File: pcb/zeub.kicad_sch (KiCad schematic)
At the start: 39 parts, among them J1 debug-port, J2 OLED-128x32, J5 Conn_01x03, J6 Conn_01x03, J7 Micro_SD_Card_Det, Q1 AO3400A, Q2 AO3400A, Q3 AO3400A, Q4 AO3400A, Q5 AO3400A, Q6 AO3401A, Q7 AO3401A, Q8 AO3401A, Q9 AO3401A, SW1 SKRHA, SW2 RotaryEncoder_Switch, SW3 SW_Push, U11 TMP117, U5 holyiot-18010-no-underside, U6 MT25QL128ABA1ESE

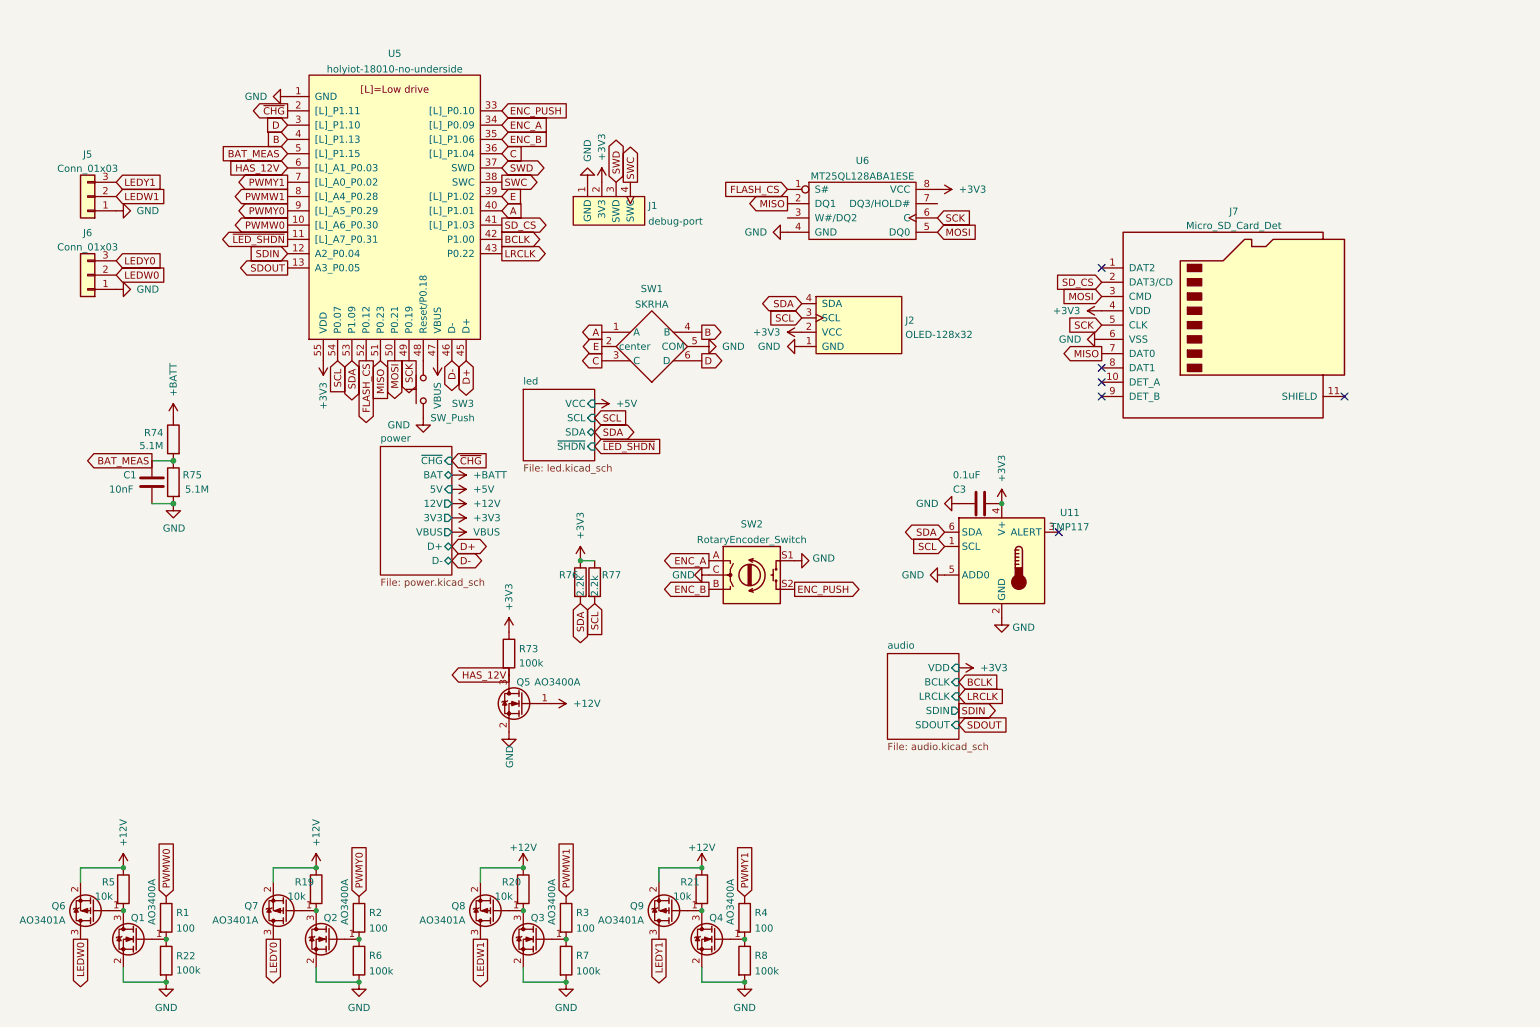
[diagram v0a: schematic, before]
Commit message: v2
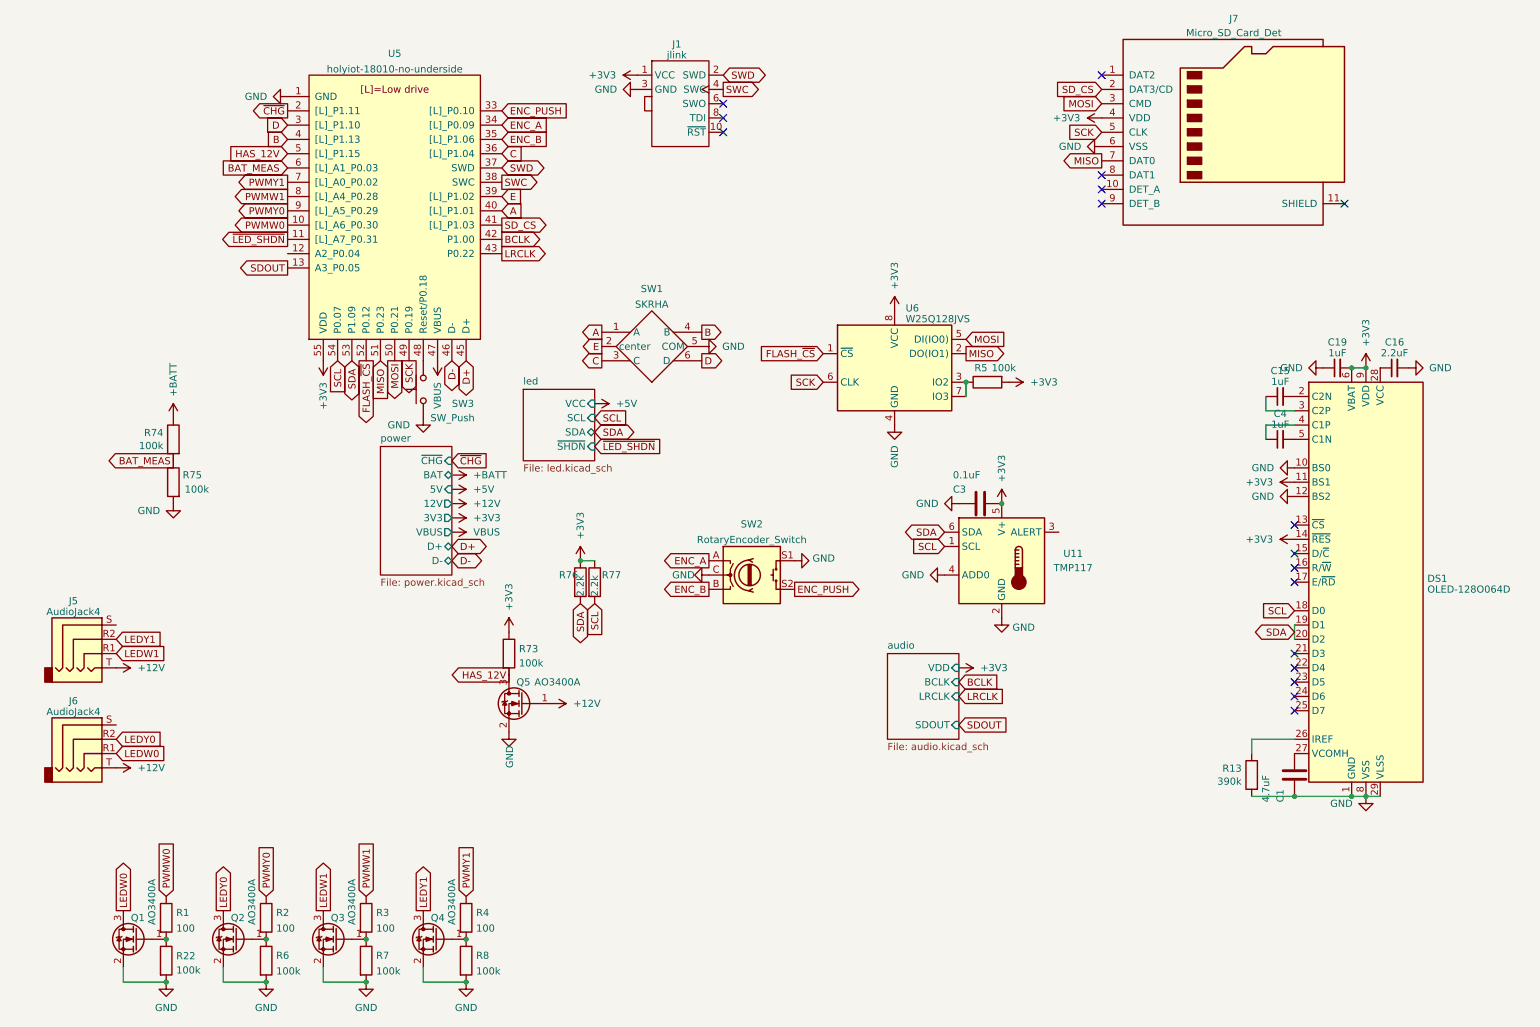
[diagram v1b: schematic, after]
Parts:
- removed J1: debug-port, misc:debug-port-single-side, symbol misc:debug-port
- removed J2: OLED-128x32, display:OLED-128x64, symbol display:OLED-128x32
- removed J5, J6: Conn_01x03, Connector_PinHeader_2.54mm:PinHeader_1x03_P2.54mm_Vertical, symbol Connector_Generic:Conn_01x03
- removed Q6, Q7, Q8, Q9: AO3401A, Package_TO_SOT_SMD:SOT-23, symbol Transistor_FET:AO3401A
- removed R19, R20, R21: 10k, Resistor_SMD:R_0603_1608Metric, symbol Device:R
- removed U6: MT25QL128ABA1ESE, Package_SO:SOIC-8_5.23x5.23mm_P1.27mm, symbol ic:MT25QL128ABA1ESE
- added C15, C19, C4: 1uF, Capacitor_SMD:C_0603_1608Metric, symbol Device:C_Small
- added C16: 2.2uF, Capacitor_SMD:C_0603_1608Metric, symbol Device:C_Small
- added DS1: OLED-128O064D, Display:OLED-128O064D, symbol Display_Graphic:OLED-128O064D
- added J1: jlink, Connector_PinHeader_1.27mm:PinHeader_2x05_P1.27mm_Vertical_SMD, symbol misc:jlink
- added J5, J6: AudioJack4, Connector_Audio:Jack_3.5mm_PJ320D_Horizontal, symbol Connector:AudioJack4
- added R13: 390k, Resistor_SMD:R_0603_1608Metric, symbol Device:R
- added U6: W25Q128JVS, Package_SO:SOIC-8_5.23x5.23mm_P1.27mm, symbol Memory_Flash:W25Q128JVS
- C1: value 10nF -> 4.7uF
- R5: value 10k -> 100k
- R74, R75: value 5.1M -> 100k
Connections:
- net +12V: now also J5.T, J6.T; no longer R5.1
- net +3V3: now also R5.2, U11.5 (V+), C19.2, DS1.11 (BS1), DS1.14 (~{RES}), DS1.6 (VBAT), DS1.9 (VDD), J1.1 (VCC), U6.8 (VCC); no longer U11.4 (V+)
- net BAT_MEAS: now also U5.6 ([L]_A1_P0.03); no longer C1.1, U5.5 ([L]_P1.15)
- net GND: now also C1.1, U11.4 (ADD0), C16.2, C19.1, DS1.1 (GND), DS1.10 (BS0), DS1.12 (BS2), DS1.29 (VLSS), DS1.30 (GND), DS1.8 (VSS), J1.3 (GND), J1.5 (GND), R13.2, U6.4 (GND); no longer C1.2, U11.5 (ADD0)
- net HAS_12V: now also U5.5 ([L]_P1.15); no longer U5.6 ([L]_A1_P0.03)
- net LEDW0: now also Q1.3 (D), J6.R1
- net LEDW1: now also Q3.3 (D), J5.R1
- net LEDY0: now also Q2.3 (D), J6.R2
- net LEDY1: now also Q4.3 (D), J5.R2
- net MISO: now also U6.2 (DO(IO1))
- net MOSI: now also U6.5 (DI(IO0))
- net SCK: now also U6.6 (CLK)
- net SCL: now also DS1.18 (D0)
- net SDA: now also DS1.19 (D1), DS1.20 (D2)
- net SWC: now also J1.4 (SWC)
- net SWD: now also J1.2 (SWD)
- net FLASH_CS renamed FLASH_~{CS}
- net FLASH_~{CS}: now also U6.1 (~{CS})
- net SDIN: no longer names the net of U5.12 (A2_P0.04)
- new net: R5.1, U6.3 (IO2), U6.7 (IO3)
- new net: C4.1, DS1.4 (C1P)
- new net: C4.2, DS1.5 (C1N)
- new net: C16.1, DS1.28 (VCC)
- new net: C1.2, DS1.27 (VCOMH)
- new net: C15.1, DS1.3 (C2P)
- new net: C15.2, DS1.2 (C2N)
- new net: DS1.26 (IREF), R13.1
- no-connect marks 6 -> 17
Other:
- sheet audio ports: added none; removed SDIN
- moved on the sheet: J7, Q2, Q3, Q4, R2, R3, R4, R6, R7, R8

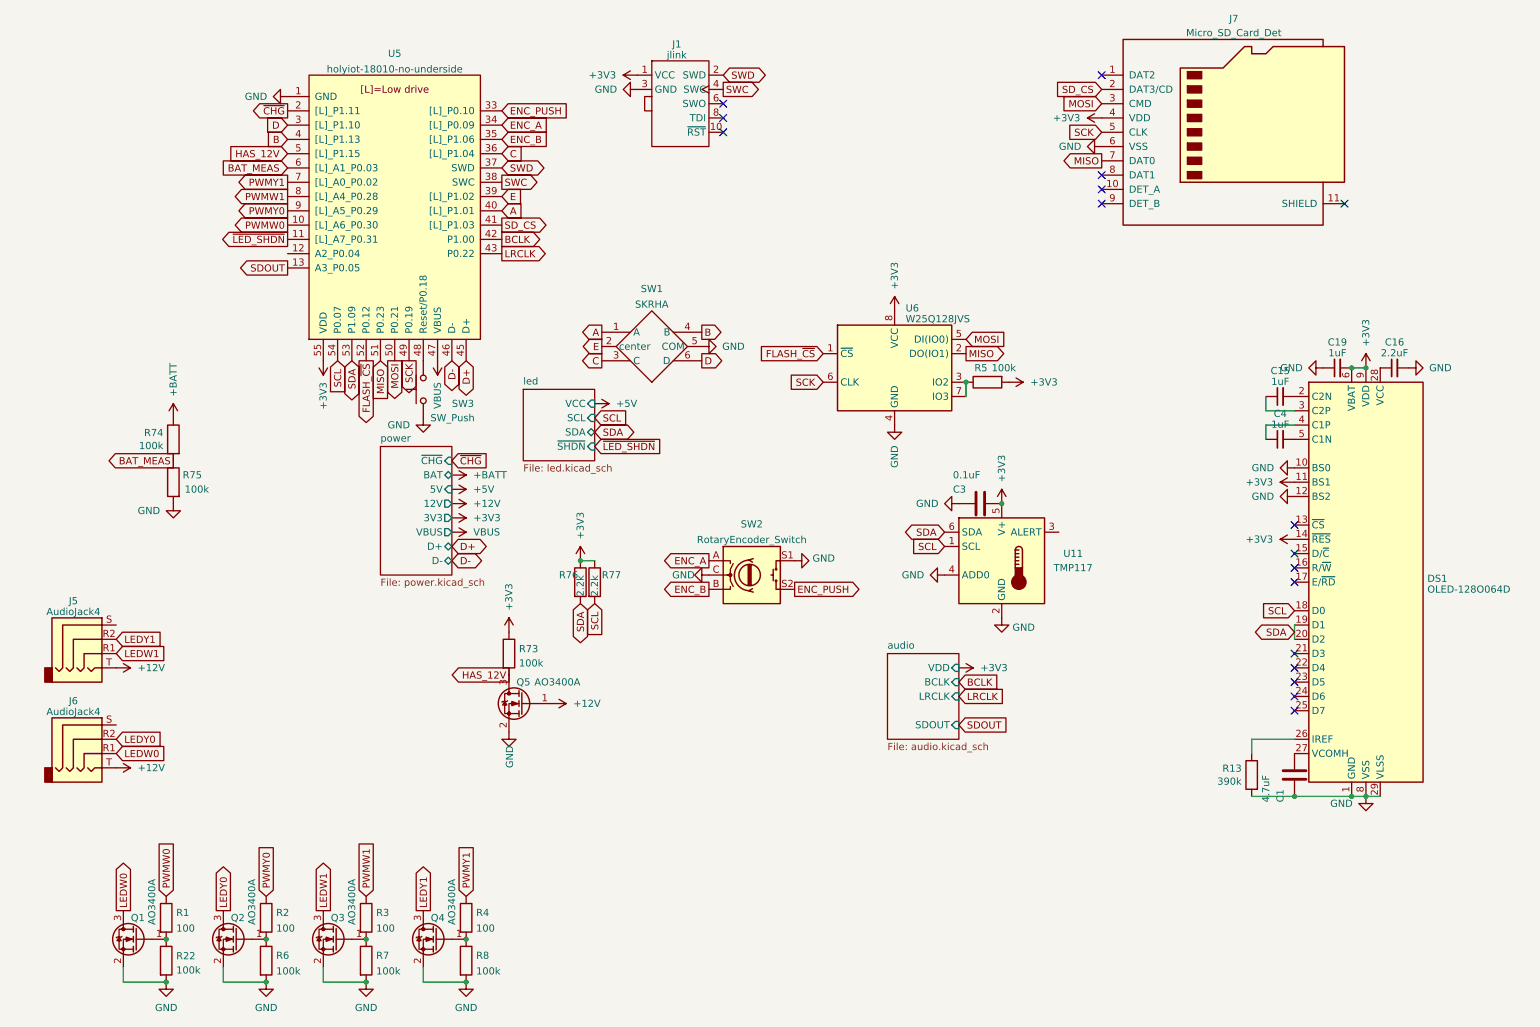
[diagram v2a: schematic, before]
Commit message: v2 fabbed
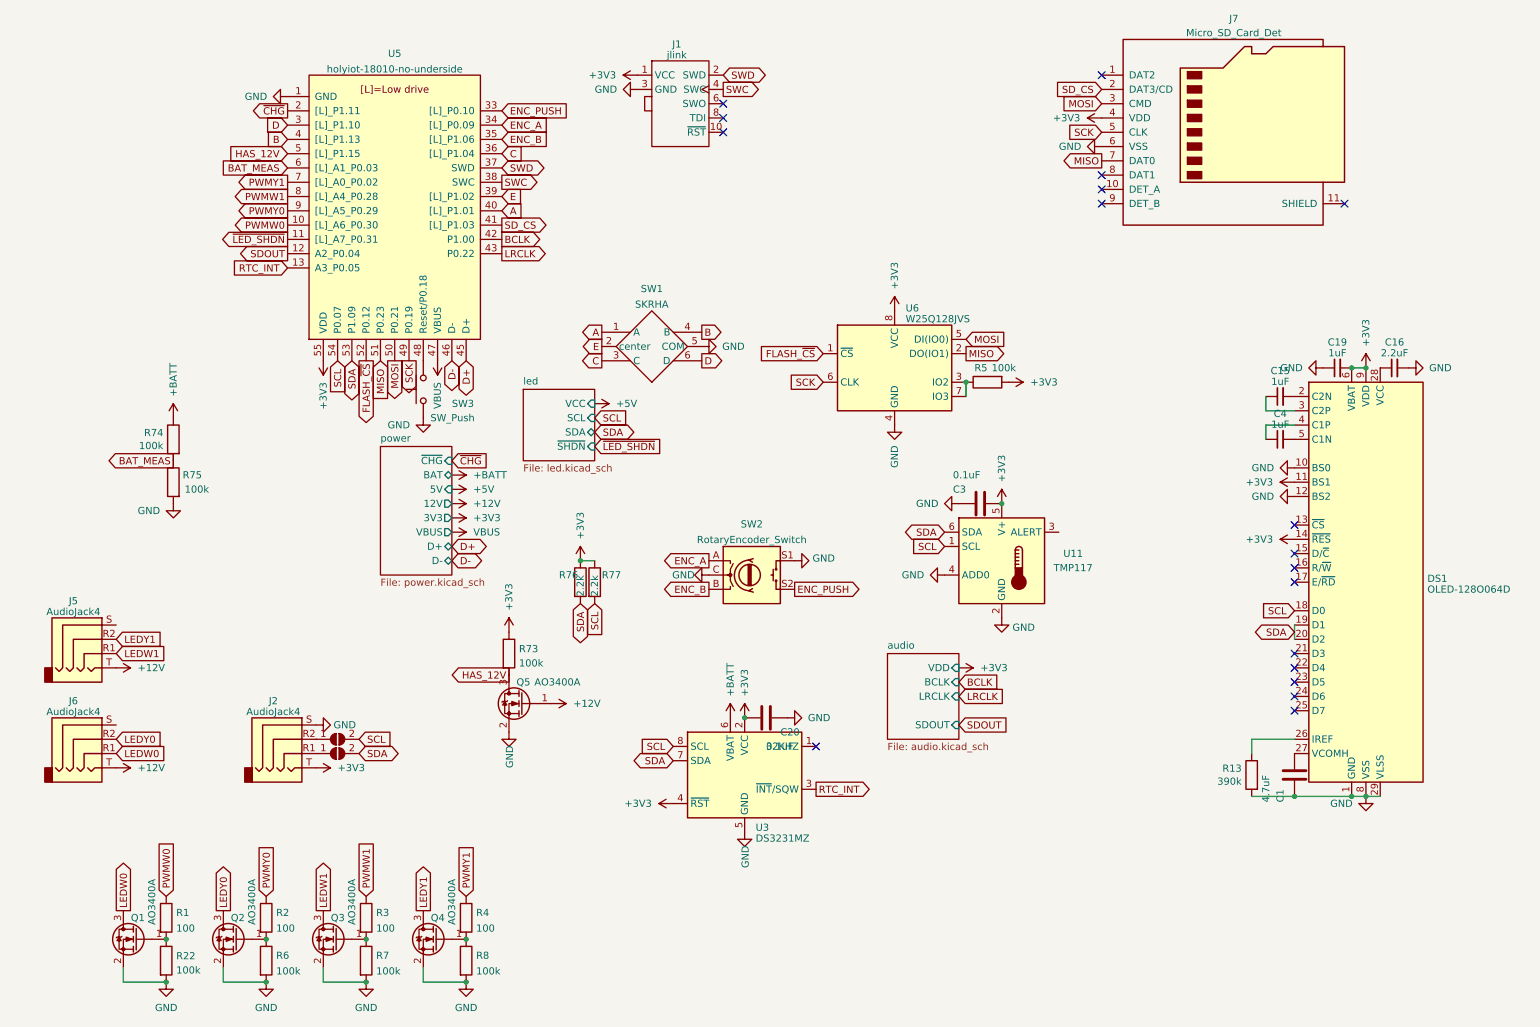
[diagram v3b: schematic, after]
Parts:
- added C20: 0.1uF, Capacitor_SMD:C_0603_1608Metric, symbol Device:C
- added J2: AudioJack4, Connector_Audio:Jack_3.5mm_PJ320D_Horizontal, symbol Connector:AudioJack4
- added JP3, JP4: SolderJumper_2_Open, Jumper:SolderJumper-2_P1.3mm_Open_TrianglePad1.0x1.5mm, symbol Jumper:SolderJumper_2_Open
- added U3: DS3231MZ, Package_SO:SOIC-8_3.9x4.9mm_P1.27mm, symbol Timer_RTC:DS3231MZ
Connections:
- net +3V3: now also C20.2, J2.T, U3.2 (VCC), U3.4 (~{RST})
- net +BATT: now also U3.6 (VBAT)
- net GND: now also C20.1, J2.S, U3.5 (GND)
- net SCL: now also JP4.2 (B), U3.8 (SCL)
- net SDA: now also JP3.2 (B), U3.7 (SDA)
- net SDOUT: now also U5.12 (A2_P0.04); no longer U5.13 (A3_P0.05)
- new net: J2.R1, JP3.1 (A)
- new net: J2.R2, JP4.1 (A)
- new net RTC_INT: U3.3 (~{INT}/SQW), U5.13 (A3_P0.05)
- no-connect marks 17 -> 18
